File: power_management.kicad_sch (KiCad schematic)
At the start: 34 parts, among them J1 705510001, Q1 SSM3J327R, U18 TPS2117DRL, U6 TLV840MADL22DBVR, U7 TPS22917DBV, U8 OPA333 or TLV333 or TLV9041

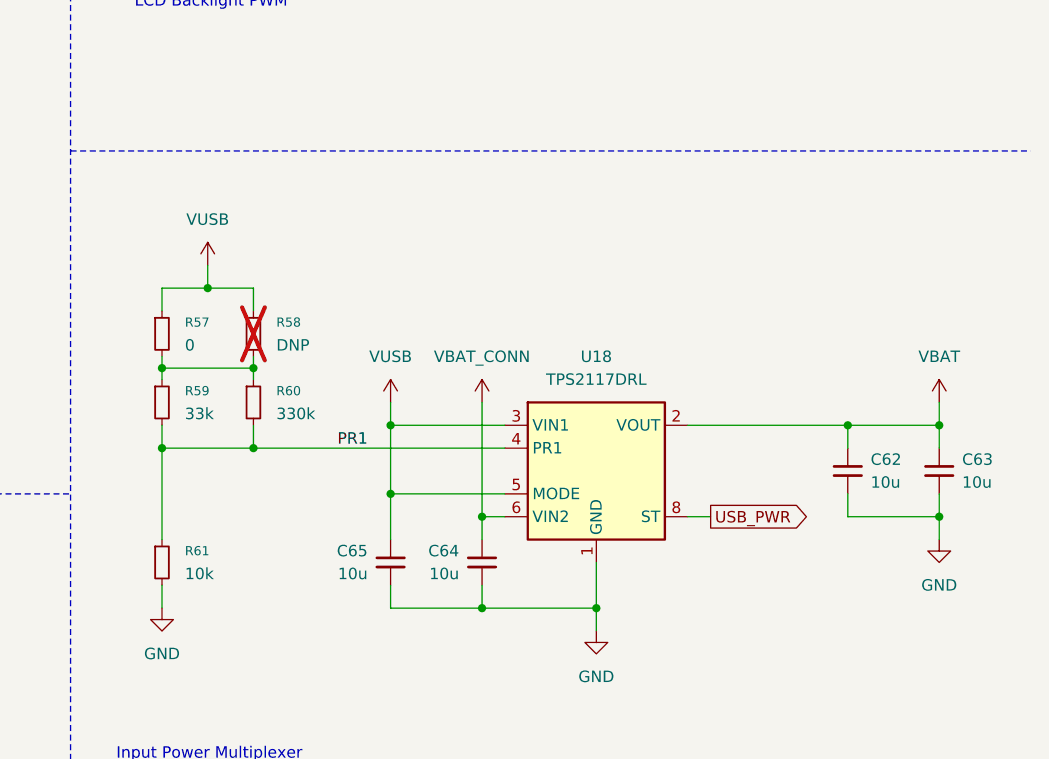
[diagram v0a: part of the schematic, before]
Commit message: Final version sent for fabrication
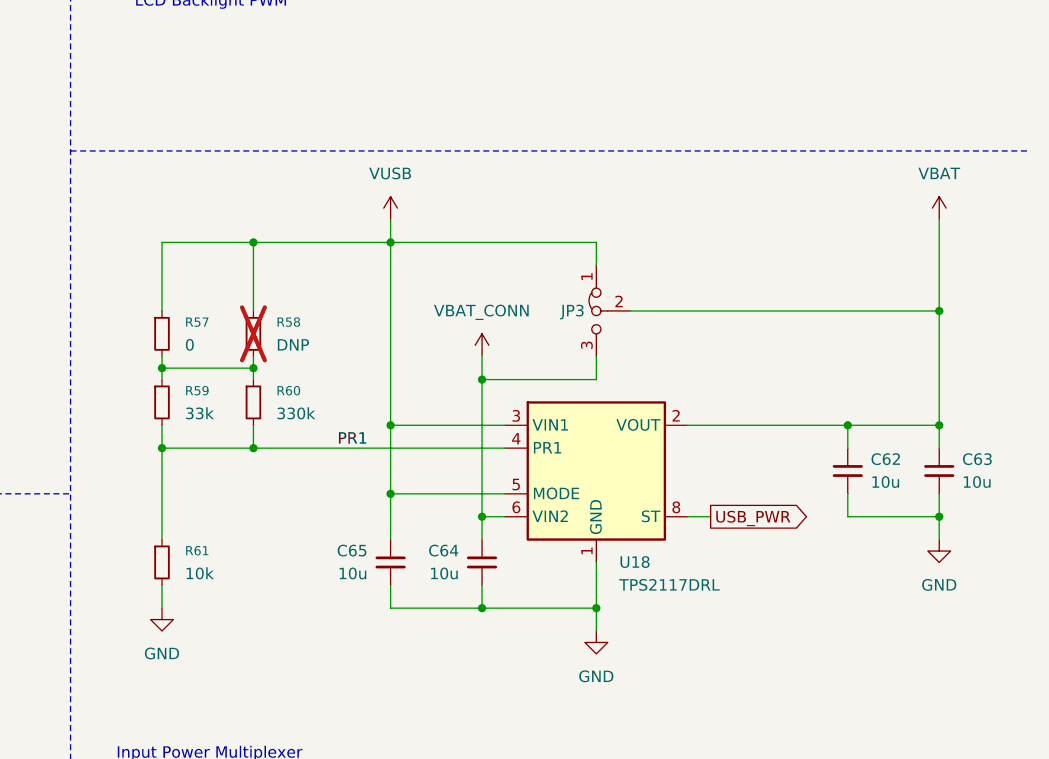
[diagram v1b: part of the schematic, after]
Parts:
- added JP3: Jumper_3_Bridged12, Connector_PinHeader_2.54mm:PinHeader_1x03_P2.54mm_Vertical, symbol Jumper:Jumper_3_Bridged12
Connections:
- net VBAT: now also JP3.2 (C)
- net VBAT_CONN: now also JP3.3 (B)
- net VUSB: now also JP3.1 (A)
